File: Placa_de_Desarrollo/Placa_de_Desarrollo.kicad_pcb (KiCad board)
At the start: 2 copper layers, 97.2 x 104.8 mm, 30 parts, among them J1 USB_A, J2 LEFT, J3 RIGHT, SW1 RESET, U1 LM317_TO-220, U2 RP2350

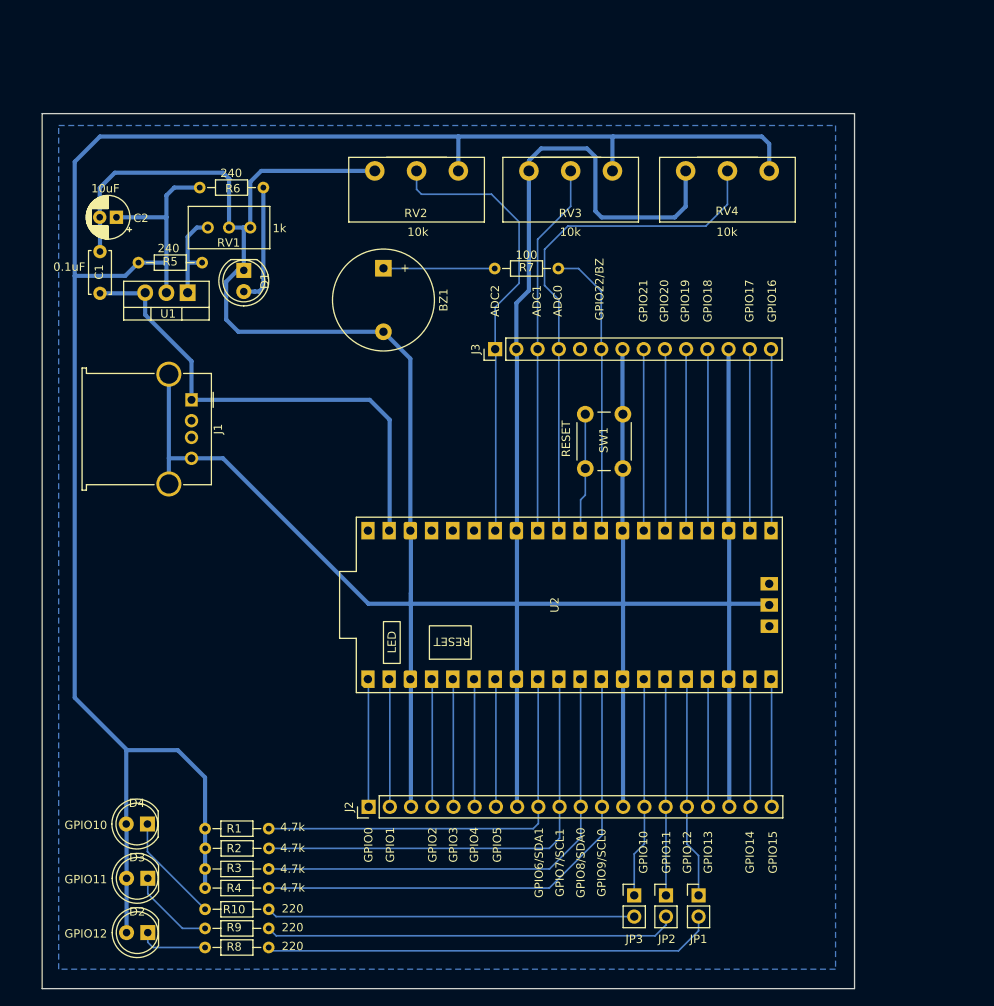
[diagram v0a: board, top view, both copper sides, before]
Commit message: Version 2.0 de la Placa de DEsarrollo
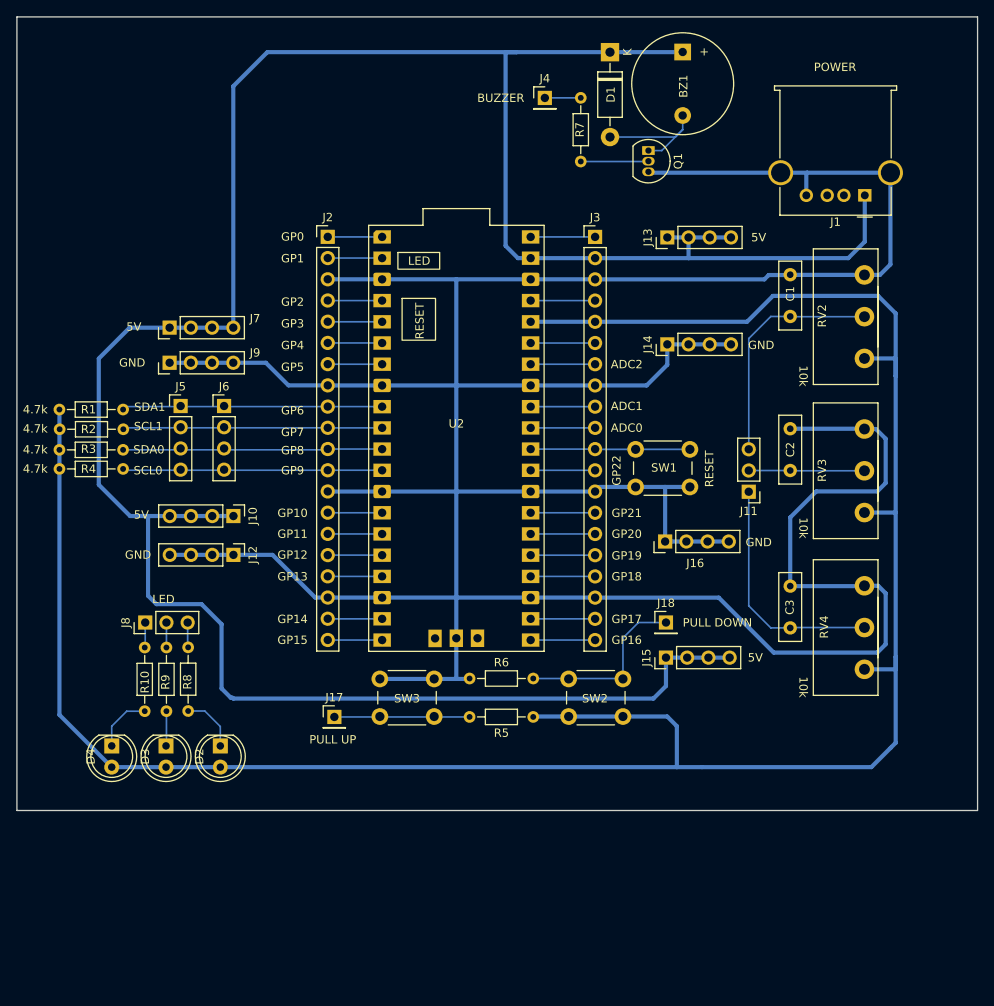
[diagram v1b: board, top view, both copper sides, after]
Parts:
- removed JP1, JP2, JP3: Jumper_2_Bridged, Connector_PinHeader_2.54mm:PinHeader_1x02_P2.54mm_Vertical
- removed RV1: 1K, Potentiometer_THT:Potentiometer_Bourns_3296W_Vertical
- removed U1: LM317_TO-220, Package_TO_SOT_THT:TO-220-3_Vertical
- added C3: 100nF, Capacitor_THT:C_Disc_D8.0mm_W2.5mm_P5.00mm, F.Cu at (198.6, 98.1)
- added J10: Conn_01x04, Connector_PinHeader_2.54mm:PinHeader_1x04_P2.54mm_Vertical, F.Cu at (131.9, 84.8)
- added J11: Conn_01x03, Connector_PinHeader_2.54mm:PinHeader_1x03_P2.54mm_Vertical, F.Cu at (193.6, 81.8)
- added J12: Conn_01x04, Connector_PinHeader_2.54mm:PinHeader_1x04_P2.54mm_Vertical, F.Cu at (131.9, 89.4)
- added J13: Conn_01x04, Connector_PinHeader_2.54mm:PinHeader_1x04_P2.54mm_Vertical, F.Cu at (183.9, 51.4)
- added J14: Conn_01x04, Connector_PinHeader_2.54mm:PinHeader_1x04_P2.54mm_Vertical, F.Cu at (183.9, 64.2)
- added J15: Conn_01x04, Connector_PinHeader_2.54mm:PinHeader_1x04_P2.54mm_Vertical, F.Cu at (183.7, 101.7)
- added J16: Conn_01x04, Connector_PinHeader_2.54mm:PinHeader_1x04_P2.54mm_Vertical, F.Cu at (183.6, 87.8)
- added J17: Conn_01x01, Connector_PinHeader_2.54mm:PinHeader_1x01_P2.54mm_Vertical, F.Cu at (144.0, 108.8)
- added J18: Conn_01x01, Connector_PinHeader_2.54mm:PinHeader_1x01_P2.54mm_Vertical, F.Cu at (183.7, 97.5)
- added J4: Conn_01x01, Connector_PinHeader_2.54mm:PinHeader_1x01_P2.54mm_Vertical, F.Cu at (169.2, 34.7)
- added J5: Conn_01x04, Connector_PinHeader_2.54mm:PinHeader_1x04_P2.54mm_Vertical, F.Cu at (125.6, 71.6)
- added J6: Conn_01x04, Connector_PinHeader_2.54mm:PinHeader_1x04_P2.54mm_Vertical, F.Cu at (130.8, 71.6)
- added J7: Conn_01x04, Connector_PinHeader_2.54mm:PinHeader_1x04_P2.54mm_Vertical, F.Cu at (124.3, 62.2)
- added J8: Conn_01x03, Connector_PinHeader_2.54mm:PinHeader_1x03_P2.54mm_Vertical, F.Cu at (121.4, 97.5)
- added J9: Conn_01x04, Connector_PinHeader_2.54mm:PinHeader_1x04_P2.54mm_Vertical, F.Cu at (124.3, 66.4)
- added Q1: BC547, Package_TO_SOT_THT:TO-92_Inline, F.Cu at (181.6, 41.0)
- added SW2: ´PULL DOWN, Button_Switch_THT:SW_PUSH_6mm, F.Cu at (178.6, 108.8)
- added SW3: PULL UP, Button_Switch_THT:SW_PUSH_6mm, F.Cu at (149.4, 104.2)
- C1: value 0.1uF -> 100nF; footprint Capacitor_THT:C_Disc_D5.0mm_W2.5mm_P5.00mm -> Capacitor_THT:C_Disc_D8.0mm_W2.5mm_P5.00mm
- C2: value 10uF -> 100nF; footprint Capacitor_THT:CP_Radial_D5.0mm_P2.00mm -> Capacitor_THT:C_Disc_D8.0mm_W2.5mm_P5.00mm
- D1: value LED -> 1N4007; footprint LED_THT:LED_D5.0mm -> Diode_THT:D_DO-41_SOD81_P10.16mm_Horizontal
- J3: footprint Connector_PinHeader_2.54mm:PinHeader_1x14_P2.54mm_Vertical -> Connector_PinHeader_2.54mm:PinHeader_1x20_P2.54mm_Vertical
- R5, R6: value 240 -> 10K
- R7: value 100 -> 1K
- moved C2 86.2 mm to (198.6, 79.3), turned to 90 degrees
- moved J1 84.2 mm to (207.5, 46.4), turned to 180 degrees
- moved C1 82.7 mm to (198.6, 60.9)
- moved J2 68.4 mm to (143.2, 51.3), turned to 0 degrees
- moved R5 67.3 mm to (167.8, 108.8)
- moved R6 67.1 mm to (160.2, 104.2)
- moved RV4 60.7 mm to (207.5, 103.1), turned to 0 degrees
- moved RV2 53.5 mm to (207.5, 65.9), turned to 0 degrees
- moved R1 53.1 mm to (111.1, 72.0)
- moved R3 53.1 mm to (111.1, 76.8)
- moved R4 53.1 mm to (111.1, 79.1)
- moved R2 53.1 mm to (111.1, 74.4)
- moved D1 51.0 mm to (177.0, 29.2)
- moved RV3 50.8 mm to (207.5, 84.3), turned to 0 degrees
- moved BZ1 44.2 mm to (185.7, 29.2)
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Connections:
- net LED1 renamed GPIO10
- net LED2 renamed GPIO11
- net LED3 renamed GPIO12
- BZ1 pad 1: Net-(BZ1-+) -> 5V
- BZ1 pad 2: GND -> Net-(BZ1--)
- C1 pad 1: 5V -> ADC0
- C2 pad 1: 3.3V -> ADC1
- D1 pad 1: GND -> 5V
- D1 pad 2: Net-(D1-A) -> Net-(BZ1--)
- J3 pad 1: ADC2 -> VBUS
- J3 pad 10: GPIO19 -> GPIO26
- J3 pad 11: GPIO18 -> RESET
- J3 pad 12: GND -> GPIO22
- J3 pad 13: GPIO17 -> GND
- J3 pad 14: GPIO16 -> GPIO21
- J3 pad 2: GND -> 5V
- J3 pad 3: ADC1 -> GND
- J3 pad 4: ADC0 -> 3V3_EB
- J3 pad 5: unconnected-(J3-Pin_5-Pad5) -> 3.3V
- J3 pad 6: BUZZER -> ADC_REF
- J3 pad 7: GND -> GPIO28
- J3 pad 8: GPIO21 -> GND
- J3 pad 9: GPIO20 -> GPIO27
- R5 pad 1: Net-(U1-ADJ) -> 3.3V
- R5 pad 2: 3.3V -> Net-(J17-Pin_1)
- R6 pad 1: 3.3V -> GND
- R6 pad 2: Net-(D1-A) -> Net-(J18-Pin_1)
- R7 pad 1: BUZZER -> Net-(J4-Pin_1)
- R7 pad 2: Net-(BZ1-+) -> Net-(Q1-B)
- RV2 pad 2: ADC2 -> ADC0
- RV4 pad 2: ADC0 -> ADC2
- SW1 pad 1: Net-(U2-RUN) -> RESET
- U2 pad 29: BUZZER -> GPIO22
- U2 pad 30: Net-(U2-RUN) -> RESET
- U2 pad 31: ADC0 -> GPIO26
- U2 pad 32: ADC1 -> GPIO27
- U2 pad 34: ADC2 -> GPIO28
- U2 pad 35: unconnected-(U2-ADC_REF-Pad35) -> ADC_REF
- U2 pad 36: unconnected-(U2-3V3_OUT-Pad36) -> 3.3V
- U2 pad 37: unconnected-(U2-3V3_EB-Pad37) -> 3V3_EB
- U2 pad 40: unconnected-(U2-VBUS-Pad40) -> VBUS
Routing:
- net 5V: track 58.4 -> 312.1 mm
- net Net-(J8-Pin_3): track 54.3 -> 2.99 mm
- net Net-(J8-Pin_2): track 49.5 -> 2.99 mm
- net Net-(J8-Pin_1): track 44.1 -> 3.01 mm
- net BUZZER: track 34.8 -> 0.00 mm
- net ADC0: track 62.4 -> 28.2 mm
- net ADC1: track 44.6 -> 13.9 mm
- net SCL0: track 61.3 -> 31.1 mm
- net SDA0: track 58.0 -> 31.1 mm
- net 3.3V: track 248.9 -> 275.1 mm
- net ADC2: track 54.1 -> 28.6 mm
- net SCL1: track 54.4 -> 31.1 mm
- net Net-(J18-Pin_1): track 0.00 -> 21.6 mm
- net GPIO12: track 26.6 -> 6.51 mm
- net GPIO10: track 26.5 -> 6.51 mm
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- removed copper zone on B.Cu, net GND
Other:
- board size 97.2 x 104.8 mm -> 115 x 95 mm
- board text added: "5V"
- board text added: "BUZZER"
- board text added: "GND"
- board text added: "GP0"
- board text added: "GP1"
- board text added: "GP10"
- board text added: "GP11"
- board text added: "GP12"
- board text added: "GP13"
- board text added: "GP14"
- board text added: "GP15"
- board text added: "GP16"
- board text added: "GP17"
- board text added: "GP18"
- board text added: "GP19"
- board text added: "GP2"
- board text added: "GP20"
- board text added: "GP21"
- board text added: "GP22"
- board text added: "GP3"
- board text added: "GP4"
- board text added: "GP5"
- board text added: "GP6"
- board text added: "GP7"
- board text added: "GP8"
- board text added: "GP9"
- board text added: "LED"
- board text added: "POWER"
- board text added: "PULL DOWN"
- board text added: "PULL UP"
- board text added: "SCL0"
- board text added: "SCL1"
- board text added: "SDA0"
- board text added: "SDA1"
- board text removed: "0.1uF"
- board text removed: "100"
- board text removed: "10uF"
- board text removed: "1k"
- board text removed: "220"
- board text removed: "240"
- board text removed: "GPIO0"
- board text removed: "GPIO1"
- board text removed: "GPIO10"
- board text removed: "GPIO11"
- board text removed: "GPIO12"
- board text removed: "GPIO13"
- board text removed: "GPIO14"
- board text removed: "GPIO15"
- board text removed: "GPIO16"
- board text removed: "GPIO17"
- board text removed: "GPIO18"
- board text removed: "GPIO19"
- board text removed: "GPIO2"
- board text removed: "GPIO20"
- board text removed: "GPIO21"
- board text removed: "GPIO22/BZ"
- board text removed: "GPIO3"
- board text removed: "GPIO4"
- board text removed: "GPIO5"
- board text removed: "GPIO6/SDA1"
- board text removed: "GPIO7/SCL1"
- board text removed: "GPIO8/SDA0"
- board text removed: "GPIO9/SCL0"
